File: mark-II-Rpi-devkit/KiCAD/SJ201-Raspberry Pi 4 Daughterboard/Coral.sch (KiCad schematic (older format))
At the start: 11 parts, among them U2 CoralTPU

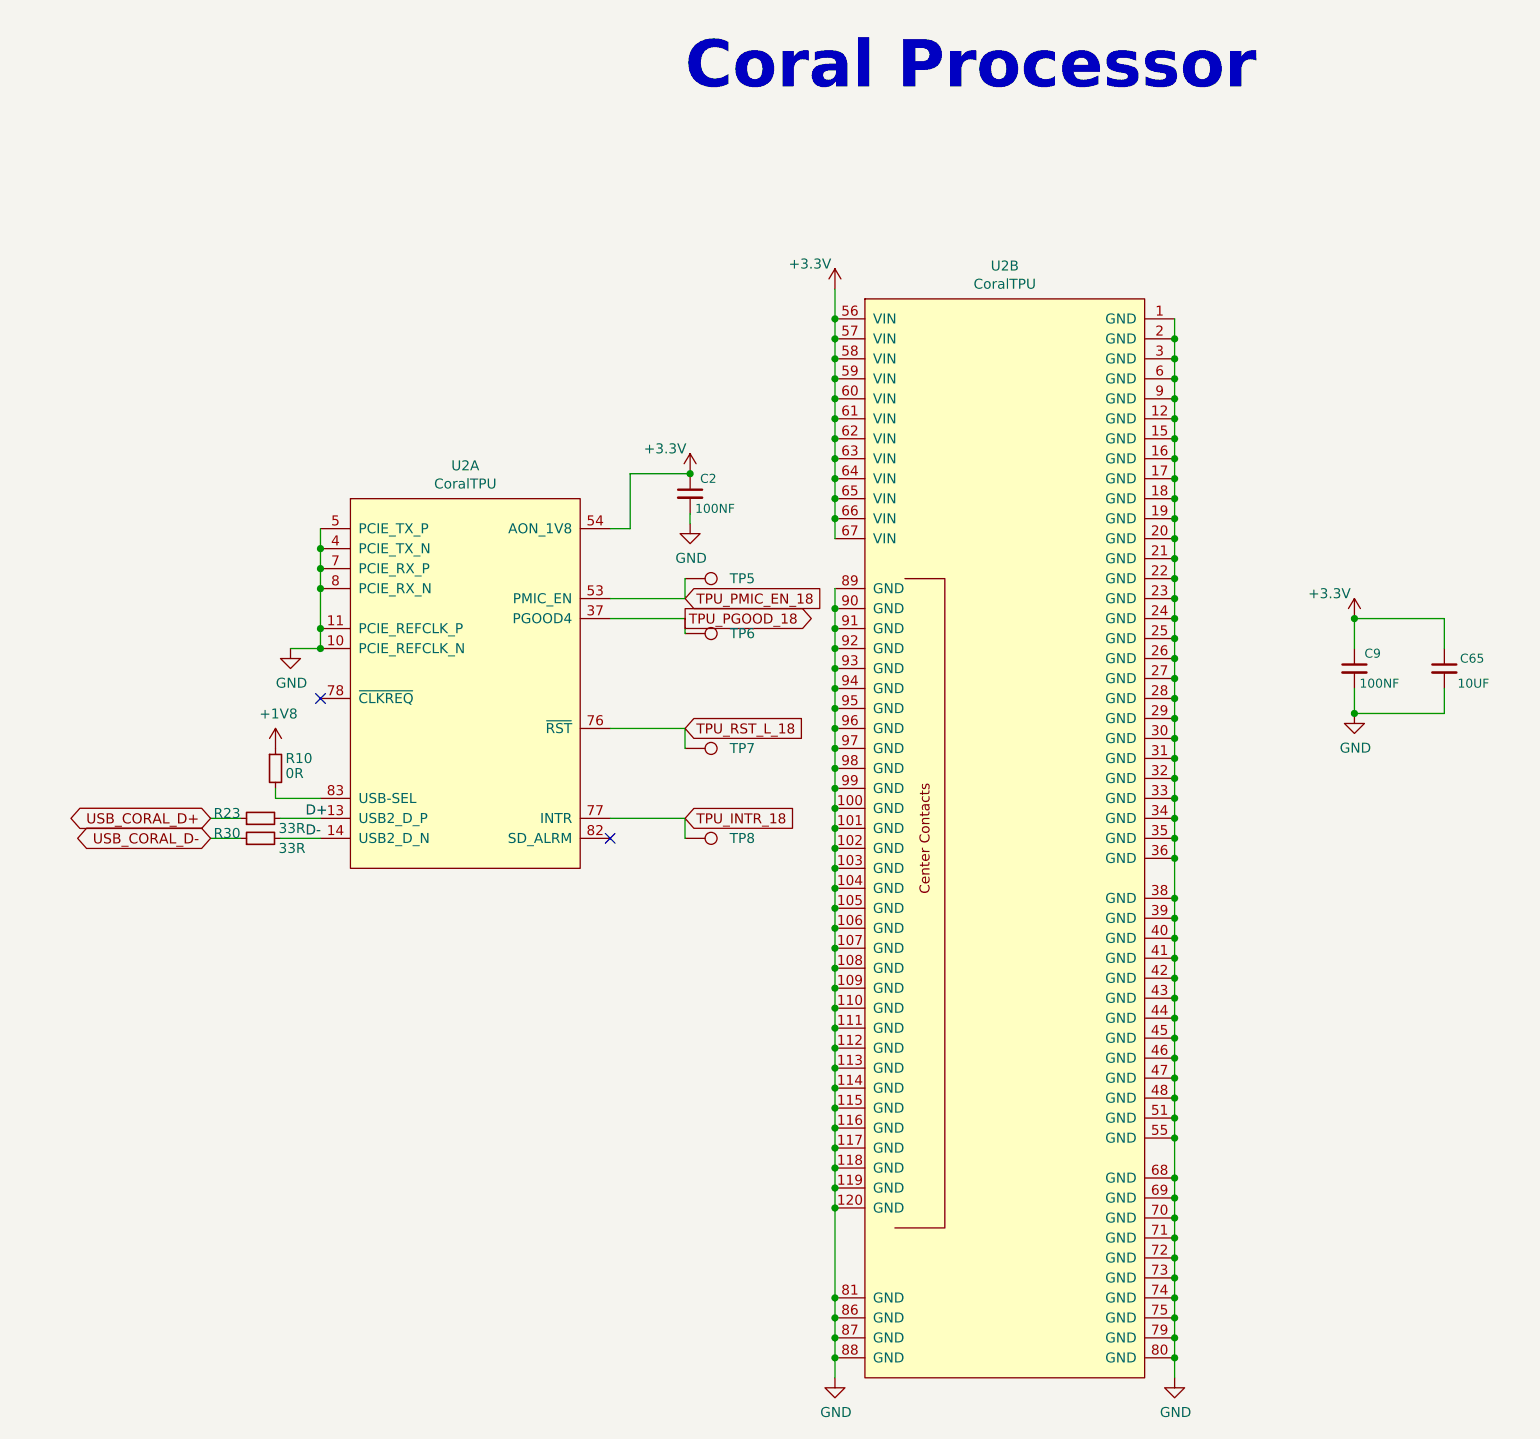
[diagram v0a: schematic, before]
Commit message: Updated files for R6 v2
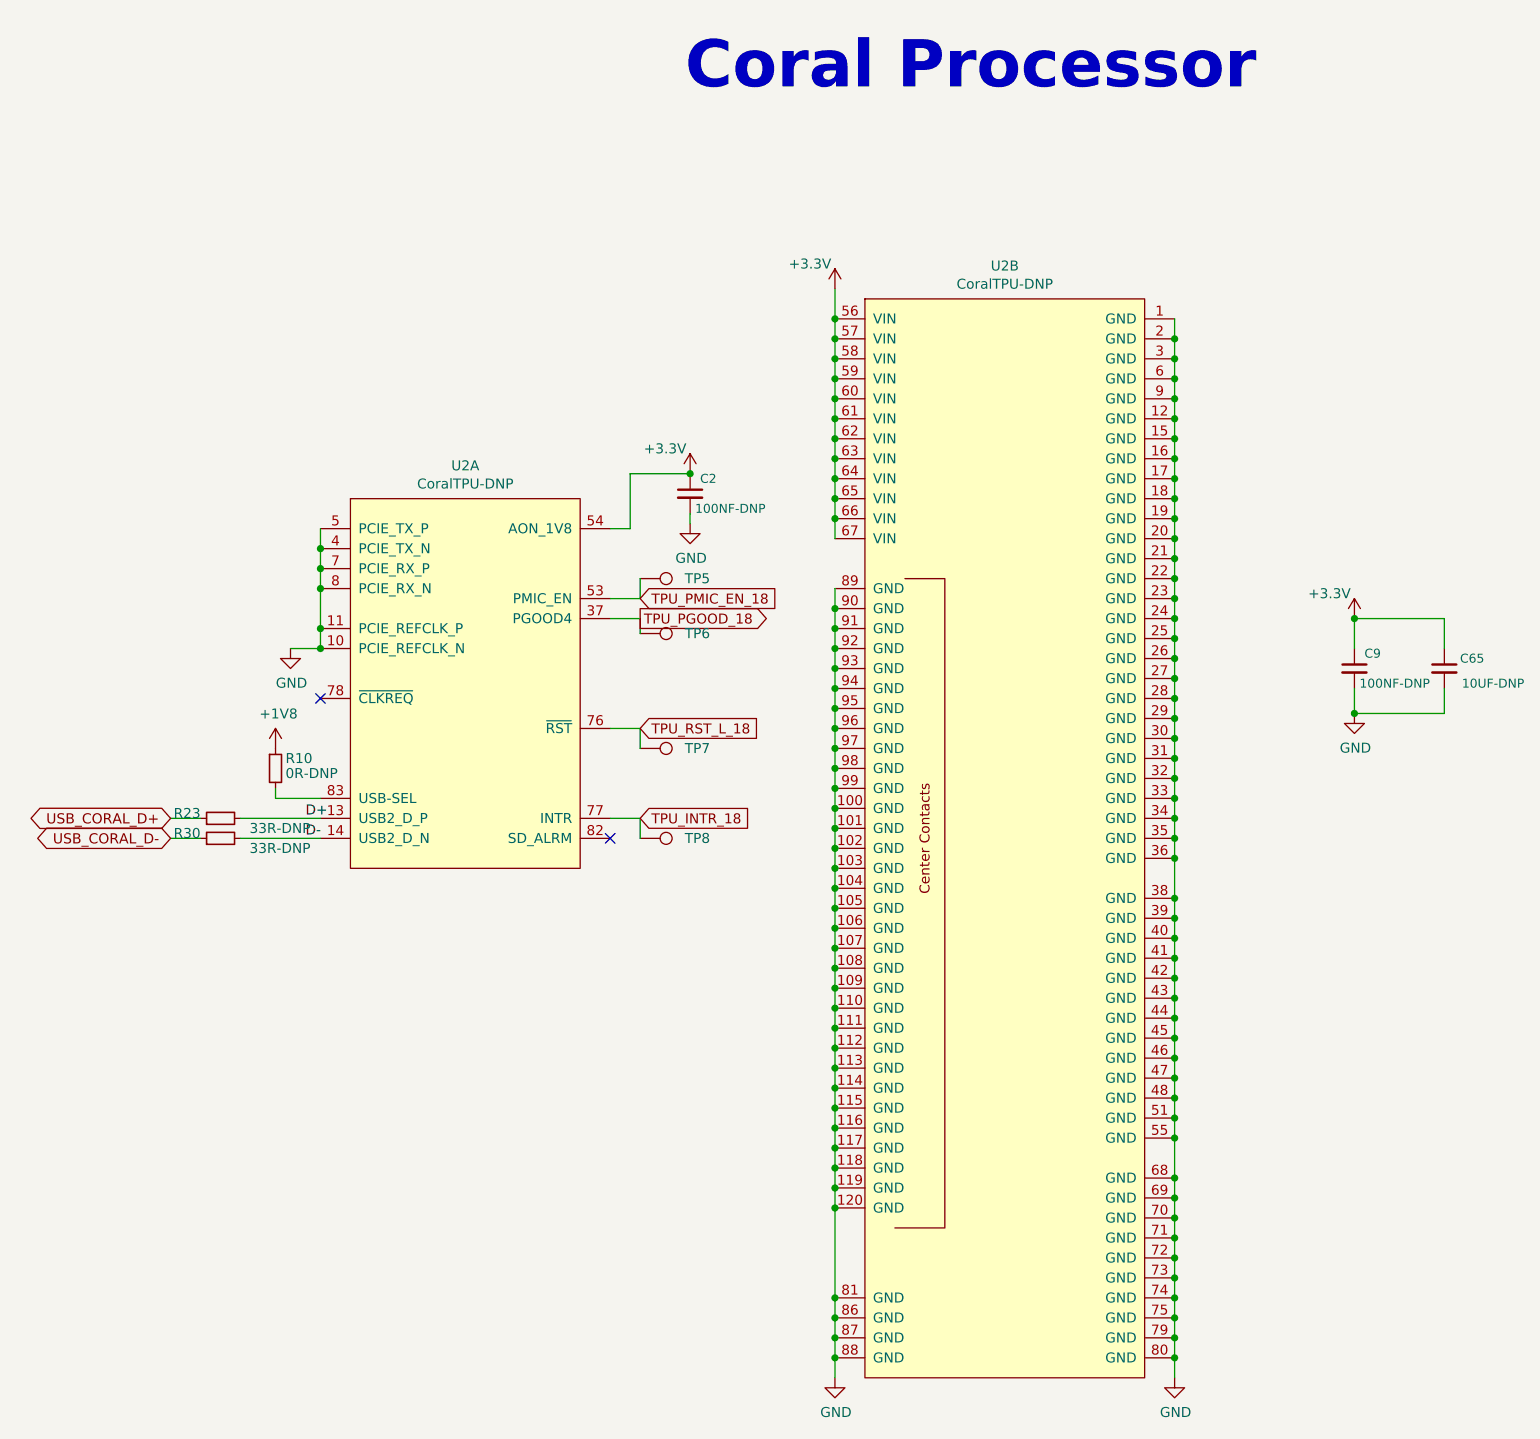
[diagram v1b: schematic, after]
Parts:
- C2, C9: value 100NF -> 100NF-DNP; LCSC C1525 -> C1525-DNP; MPN CC0402KRX7R8BB104 -> CC0402KRX7R8BB104-DNP; SKU 302010024 -> 302010024-DNP
- C65: value 10UF -> 10UF-DNP; LCSC C15525 -> C15525-DNP; MPN CC0402MRX5R5BB106 -> CC0402MRX5R5BB106-DNP; SKU 302010053 -> 302010053-DNP
- R10: value 0R -> 0R-DNP; LCSC C21189 -> C21189-DNP; MPN 0603WAF0000T5E -> 0603WAF0000T5E-DNP; Tempo RC0603JR-070RL -> RC0603JR-070RL-DNP
- R23, R30: value 33R -> 33R-DNP; LCSC C25105 -> C25105-DNP; MPN 0402WGF330JTCE -> 0402WGF330JTCE-DNP
- U2: value CoralTPU -> CoralTPU-DNP; MPN G313-06329-00 -> G313-06329-00-DNP
- U2: value CoralTPU -> CoralTPU-DNP
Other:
- moved on the sheet: R23, R30, TP5, TP6, TP7, TP8
